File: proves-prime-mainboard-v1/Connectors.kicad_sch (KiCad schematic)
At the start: 7 parts, among them J3 Conn_ARM_JTAG_SWD_10, J4 BM04B-SRSS-TB(LF)(SN), J5 USB_B_Micro

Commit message: Added USB-C Connector
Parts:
- J4: footprint FC_DEV_BOARD:JST_BM04B-SRSS-TB(LF)(SN) -> FC_DEV_BOARD:JST_BM04B-SRSS-TB(LF)(SN)
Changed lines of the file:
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@@
 			)
 		)
-		(property "Footprint" "FC_DEV_BOARD:JST_BM04B-SRSS-TB(LF)(SN) "
+		(property "Footprint" "FC_DEV_BOARD:JST_BM04B-SRSS-TB(LF)(SN)"
 			(at 83.82 38.1 0)
 			(effects

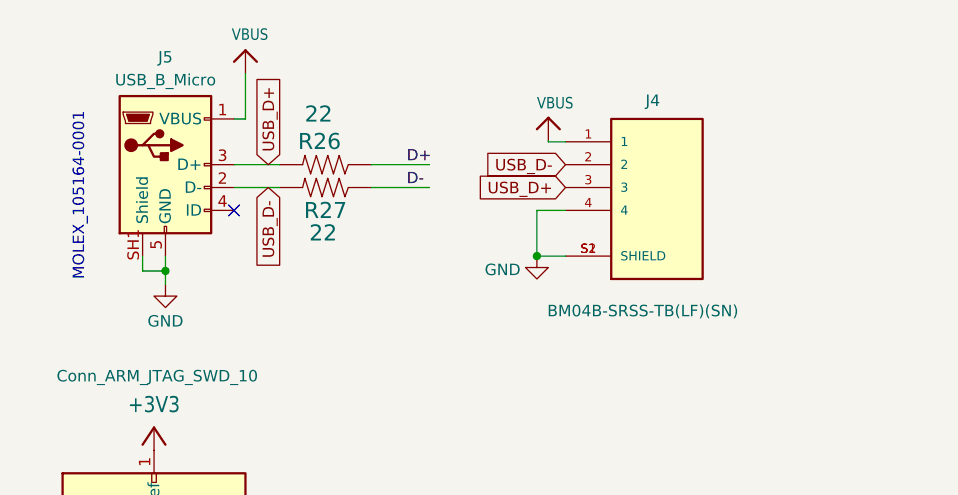
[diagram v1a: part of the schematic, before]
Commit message: More Wiring!
Connected Additional Peripheral
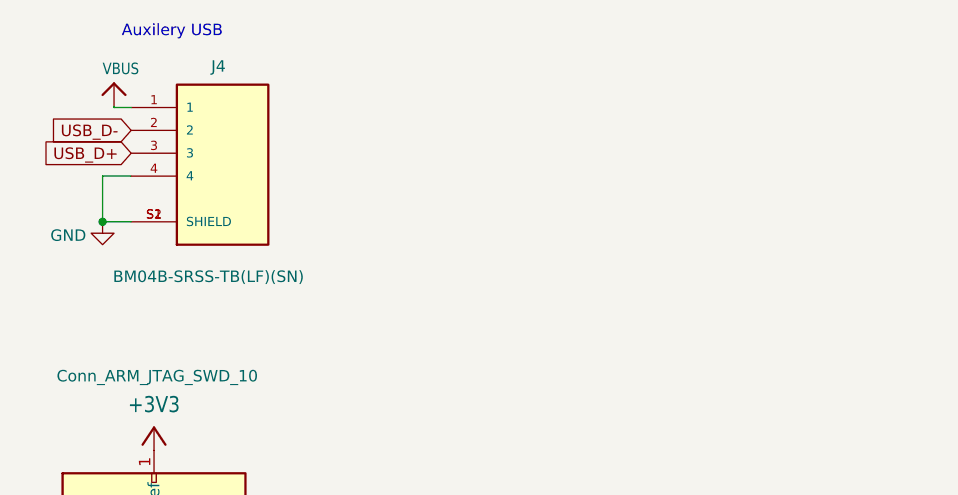
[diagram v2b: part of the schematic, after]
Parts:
- removed J5: USB_B_Micro, FC_DEV_BOARD:MOLEX_105164-0001, symbol Connector:USB_B_Micro
- removed R26, R27: 22, Resistor_SMD:R_0603_1608Metric, symbol mainboard:RESISTOR0603
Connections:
- no-connect marks 3 -> 2
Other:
- note added: "Auxilery USB"
- note removed: "MOLEX_105164-0001"
- moved on the sheet: J4
